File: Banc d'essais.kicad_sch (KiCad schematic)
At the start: 3 parts, among them U1 MCP4431-xxxx-ST

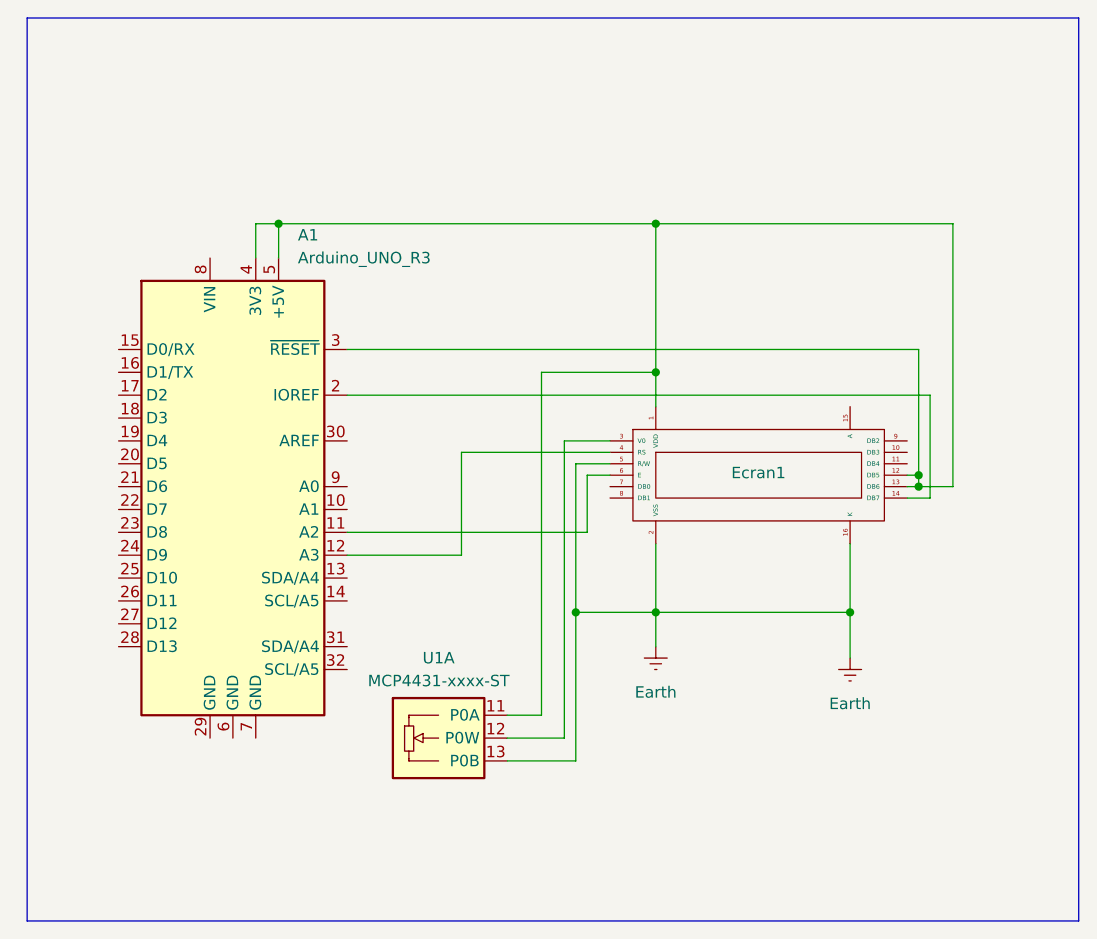
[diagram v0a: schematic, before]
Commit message: modification + finalisation du PCB et du schéma
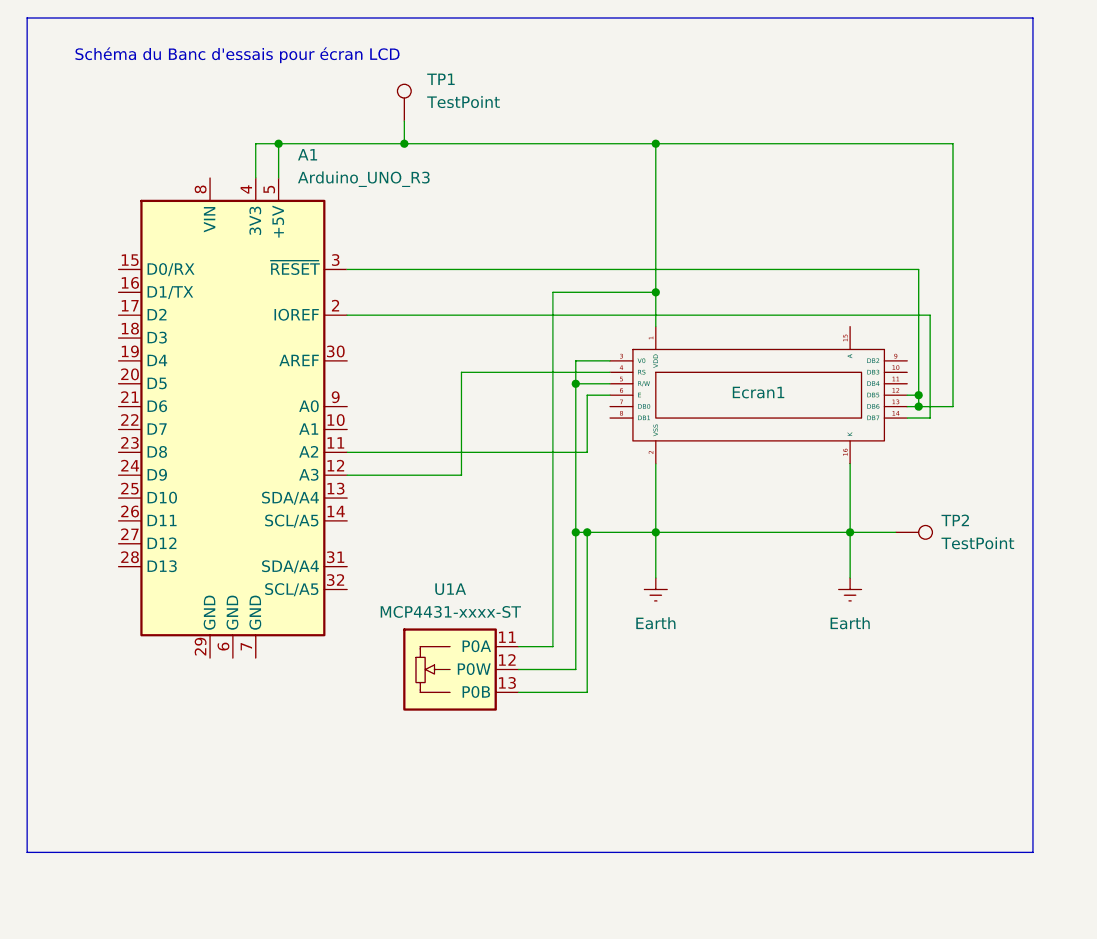
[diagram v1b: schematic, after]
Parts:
- added TP1, TP2: TestPoint, symbol Connector:TestPoint
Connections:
- net Earth: now also Ecran1.3 (V0), U1.12 (P0W), TP2.1
- net at A1.3 (~{RESET}), A1.4 (3V3), A1.5 (+5V)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: now also TP1.1
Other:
- note added: "Schéma du Banc d'essais pour écran LCD"
- moved on the sheet: A1, Ecran1, U1A
